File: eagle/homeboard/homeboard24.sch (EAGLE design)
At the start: 124 parts, among them IC1 XCF02S, IC2 25LC080SN, IC3 ATMEGA32U2-TQFP, Q5 BC848SMD, Q6 BC848SMD, Q7 BC848SMD, Q8 BC848SMD, T1 BSS138, T2 BC848, T3 BSS138, U1 XC3S400TQ144, X1 SCART-CLIP, X6 MINI-USB_4P-85-32004-10X, X7 DC21MMX, X8 STEREOJACK

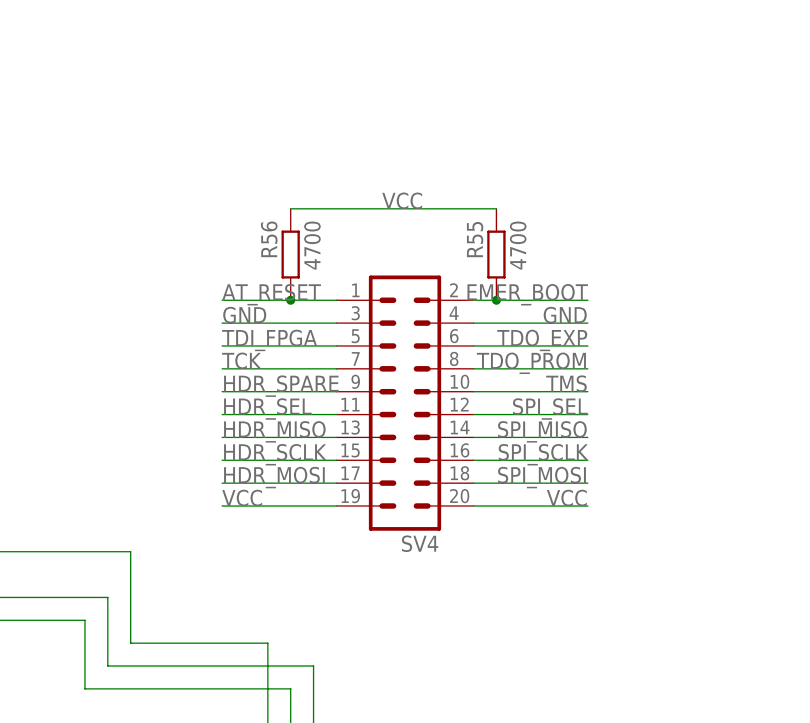
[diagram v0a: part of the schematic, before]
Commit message: moving around
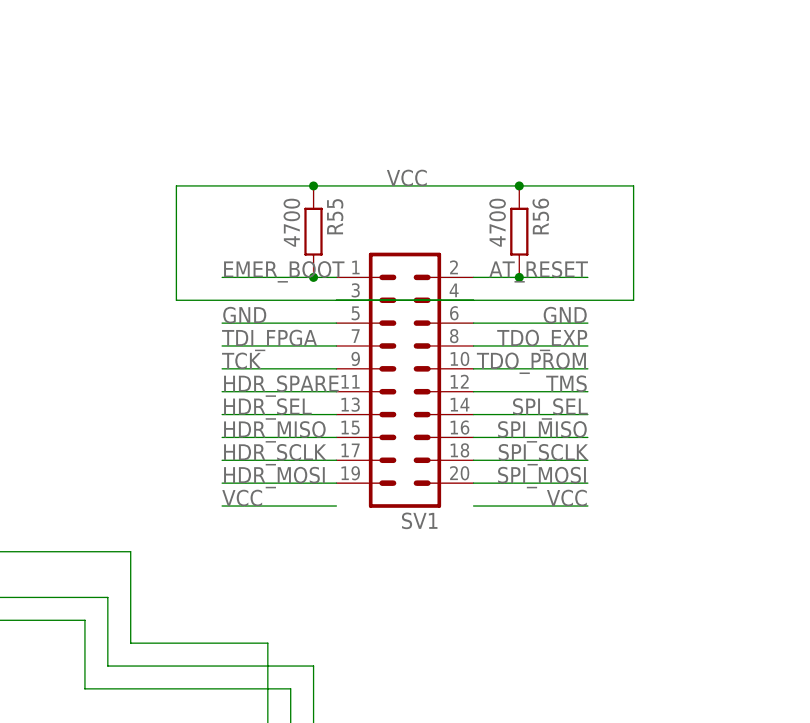
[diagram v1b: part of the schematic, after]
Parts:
- removed SV4: (no value), con-lstb:MA10-2
- added SV1: (no value), con-lstb:MA10-2
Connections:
- net AT_RESET: now also SV1.2; no longer SV4.1
- net EMER_BOOT: now also SV1.1; no longer SV4.2
- net GND: now also SV1.5, SV1.6; no longer SV4.3, SV4.4
- net HDR_MISO: now also SV1.15; no longer SV4.13
- net HDR_MOSI: now also SV1.19; no longer SV4.17
- net HDR_SCLK: now also SV1.17; no longer SV4.15
- net HDR_SEL: now also SV1.13; no longer SV4.11
- net HDR_SPARE: now also SV1.11; no longer SV4.9
- net SPI_MISO: now also SV1.16; no longer SV4.14
- net SPI_MOSI: now also SV1.20; no longer SV4.18
- net SPI_SCLK: now also SV1.18; no longer SV4.16
- net SPI_SEL: now also SV1.14; no longer SV4.12
- net TCK: now also SV1.9; no longer SV4.7
- net TDI_FPGA: now also SV1.7; no longer SV4.5
- net TDO_EXP: now also SV1.8; no longer SV4.6
- net TDO_PROM: now also SV1.10; no longer SV4.8
- net TMS: now also SV1.12; no longer SV4.10
- net VCC: now also SV1.3, SV1.4; no longer SV4.19, SV4.20
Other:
- moved on the sheet: R55, R56
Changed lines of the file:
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@@
 <part name="U$9" library="cpcfpga" deviceset="GNDHOLE" device=""/>
 <part name="SV5" library="con-lstb" deviceset="MA05-2" device=""/>
-<part name="SV4" library="con-lstb" deviceset="MA10-2" device=""/>
 <part name="JP2" library="adafruit" deviceset="PINHD-1X3" device=""/>
 <part name="SV2" library="con-lstb" deviceset="MA03-2" device=""/>
 <part name="SUPPLY16" library="supply2" deviceset="GND" device=""/>
 <part name="C13" library="rcl" deviceset="C-EU" device="C0603" value="100nF"/>
+<part name="SV1" library="con-lstb" deviceset="MA10-2" device="">
+<attribute name="MF" value=""/>
+<attribute name="MPN" value=""/>
+<attribute name="OC_FARNELL" value="unknown"/>
+<attribute name="OC_NEWARK" value="unknown"/>
+</part>
 </parts>
 <sheets>
@@
 <instance part="C41" gate="G$1" x="378.46" y="114.3" rot="R270"/>
 <instance part="SUPPLY22" gate="GND" x="373.38" y="109.22"/>
-<instance part="R55" gate="G$1" x="312.42" y="45.72" rot="MR270"/>
-<instance part="R56" gate="G$1" x="289.56" y="45.72" rot="MR270"/>
+<instance part="R55" gate="G$1" x="292.1" y="48.26" rot="R270"/>
+<instance part="R56" gate="G$1" x="314.96" y="48.26" rot="R270"/>
 <instance part="U$3" gate="G$1" x="541.02" y="40.64"/>
 <instance part="C39" gate="G$1" x="-160.02" y="109.22" smashed="yes">
@@
 <instance part="U$9" gate="G$1" x="-73.66" y="137.16"/>
 <instance part="SV5" gate="G$1" x="76.2" y="-71.12" rot="R180"/>
-<instance part="SV4" gate="G$1" x="302.26" y="30.48" rot="R180"/>
 <instance part="JP2" gate="A" x="330.2" y="119.38" rot="R90"/>
 <instance part="SV2" gate="1" x="289.56" y="-17.78" rot="R90"/>
 <instance part="SUPPLY16" gate="GND" x="292.1" y="-38.1"/>
 <instance part="C13" gate="G$1" x="-93.98" y="109.22"/>
+<instance part="SV1" gate="G$1" x="302.26" y="33.02" rot="R180"/>
 </instances>
 <busses>
@@
 <wire x1="322.58" y1="38.1" x2="309.88" y2="38.1" width="0.1524" layer="91"/>
 <label x="322.58" y="38.1" size="1.778" layer="95" rot="MR0"/>
-<pinref part="SV4" gate="G$1" pin="4"/>
+<pinref part="SV1" gate="G$1" pin="6"/>
 </segment>
 <segment>
 <wire x1="294.64" y1="38.1" x2="281.94" y2="38.1" width="0.1524" layer="91"/>
 <label x="281.94" y="38.1" size="1.778" layer="95"/>
-<pinref part="SV4" gate="G$1" pin="3"/>
+<pinref part="SV1" gate="G$1" pin="5"/>
 </segment>
 <segment>
@@
 <pinref part="R55" gate="G$1" pin="1"/>
 <pinref part="R56" gate="G$1" pin="1"/>
-<wire x1="312.42" y1="50.8" x2="289.56" y2="50.8" width="0.1524" layer="91"/>
-<label x="299.72" y="50.8" size="1.778" layer="95"/>
-</segment>
-<segment>
-<pinref part="SV4" gate="G$1" pin="19"/>
+<wire x1="292.1" y1="53.34" x2="314.96" y2="53.34" width="0.1524" layer="91"/>
+<label x="304.8" y="53.34" size="1.778" layer="95" rot="MR0"/>
+<pinref part="SV1" gate="G$1" pin="3"/>
+<wire x1="294.64" y1="40.64" x2="327.66" y2="40.64" width="0.1524" layer="91"/>
+<wire x1="327.66" y1="40.64" x2="327.66" y2="53.34" width="0.1524" layer="91"/>
+<wire x1="327.66" y1="53.34" x2="314.96" y2="53.34" width="0.1524" layer="91"/>
+<junction x="314.96" y="53.34"/>
+<pinref part="SV1" gate="G$1" pin="4"/>
+<wire x1="309.88" y1="40.64" x2="276.86" y2="40.64" width="0.1524" layer="91"/>
+<wire x1="276.86" y1="40.64" x2="276.86" y2="53.34" width="0.1524" layer="91"/>
+<wire x1="276.86" y1="53.34" x2="292.1" y2="53.34" width="0.1524" layer="91"/>
+<junction x="292.1" y="53.34"/>
+</segment>
+<segment>
 <wire x1="281.94" y1="17.78" x2="294.64" y2="17.78" width="0.1524" layer="91"/>
 <label x="281.94" y="17.78" size="1.778" layer="95"/>
 </segment>
 <segment>
-<pinref part="SV4" gate="G$1" pin="20"/>
 <wire x1="322.58" y1="17.78" x2="309.88" y2="17.78" width="0.1524" layer="91"/>
 <label x="322.58" y="17.78" size="1.778" layer="95" rot="MR0"/>
@@
 <wire x1="281.94" y1="33.02" x2="294.64" y2="33.02" width="0.1524" layer="91"/>
 <label x="281.94" y="33.02" size="1.778" layer="95"/>
-<pinref part="SV4" gate="G$1" pin="7"/>
+<pinref part="SV1" gate="G$1" pin="9"/>
 </segment>
 <segment>
@@
 <label x="322.58" y="30.48" size="1.778" layer="95" rot="MR0"/>
 <wire x1="322.58" y1="30.48" x2="309.88" y2="30.48" width="0.1524" layer="91"/>
-<pinref part="SV4" gate="G$1" pin="10"/>
+<pinref part="SV1" gate="G$1" pin="12"/>
 </segment>
 </net>
@@
 <wire x1="281.94" y1="35.56" x2="294.64" y2="35.56" width="0.1524" layer="91"/>
 <label x="281.94" y="35.56" size="1.778" layer="95"/>
-<pinref part="SV4" gate="G$1" pin="5"/>
+<pinref part="SV1" gate="G$1" pin="7"/>
 </segment>
 </net>
@@
 <segment>
 <wire x1="322.58" y1="22.86" x2="309.88" y2="22.86" width="0.1524" layer="91"/>
-<pinref part="SV4" gate="G$1" pin="16"/>
 <label x="322.58" y="22.86" size="1.778" layer="95" rot="MR0"/>
+<pinref part="SV1" gate="G$1" pin="18"/>
 </segment>
 </net>
@@
 </segment>
 <segment>
-<pinref part="SV4" gate="G$1" pin="18"/>
 <wire x1="322.58" y1="20.32" x2="309.88" y2="20.32" width="0.1524" layer="91"/>
 <label x="322.58" y="20.32" size="1.778" layer="95" rot="MR0"/>
+<pinref part="SV1" gate="G$1" pin="20"/>
 </segment>
 </net>
@@
 </segment>
 <segment>
-<pinref part="SV4" gate="G$1" pin="14"/>
 <wire x1="322.58" y1="25.4" x2="309.88" y2="25.4" width="0.1524" layer="91"/>
 <label x="322.58" y="25.4" size="1.778" layer="95" rot="MR0"/>
+<pinref part="SV1" gate="G$1" pin="16"/>
 </segment>
 </net>
@@
 <wire x1="322.58" y1="27.94" x2="309.88" y2="27.94" width="0.1524" layer="91"/>
 <label x="322.58" y="27.94" size="1.778" layer="95" rot="MR0"/>
-<pinref part="SV4" gate="G$1" pin="12"/>
+<pinref part="SV1" gate="G$1" pin="14"/>
 </segment>
 </net>
@@
 </segment>
 <segment>
-<wire x1="322.58" y1="40.64" x2="312.42" y2="40.64" width="0.1524" layer="91"/>
-<label x="322.58" y="40.64" size="1.778" layer="95" rot="MR0"/>
+<wire x1="281.94" y1="43.18" x2="292.1" y2="43.18" width="0.1524" layer="91"/>
+<label x="281.94" y="43.18" size="1.778" layer="95"/>
 <pinref part="R55" gate="G$1" pin="2"/>
-<wire x1="312.42" y1="40.64" x2="309.88" y2="40.64" width="0.1524" layer="91"/>
-<junction x="312.42" y="40.64"/>
-<pinref part="SV4" gate="G$1" pin="2"/>
+<pinref part="SV1" gate="G$1" pin="1"/>
+<wire x1="292.1" y1="43.18" x2="294.64" y2="43.18" width="0.1524" layer="91"/>
+<junction x="292.1" y="43.18"/>
 </segment>
 </net>
@@
 <wire x1="322.58" y1="33.02" x2="309.88" y2="33.02" width="0.1524" layer="91"/>
 <label x="322.58" y="33.02" size="1.778" layer="95" rot="MR0"/>
-<pinref part="SV4" gate="G$1" pin="8"/>
+<pinref part="SV1" gate="G$1" pin="10"/>
 </segment>
 </net>
@@
 <wire x1="322.58" y1="35.56" x2="309.88" y2="35.56" width="0.1524" layer="91"/>
 <label x="322.58" y="35.56" size="1.778" layer="95" rot="MR0"/>
-<pinref part="SV4" gate="G$1" pin="6"/>
+<pinref part="SV1" gate="G$1" pin="8"/>
 </segment>
 </net>
@@
 </segment>
 <segment>
-<wire x1="281.94" y1="40.64" x2="289.56" y2="40.64" width="0.1524" layer="91"/>
-<label x="281.94" y="40.64" size="1.778" layer="95"/>
+<wire x1="322.58" y1="43.18" x2="314.96" y2="43.18" width="0.1524" layer="91"/>
+<label x="322.58" y="43.18" size="1.778" layer="95" rot="MR0"/>
 <pinref part="R56" gate="G$1" pin="2"/>
-<wire x1="289.56" y1="40.64" x2="294.64" y2="40.64" width="0.1524" layer="91"/>
-<junction x="289.56" y="40.64"/>
-<pinref part="SV4" gate="G$1" pin="1"/>
+<pinref part="SV1" gate="G$1" pin="2"/>
+<wire x1="309.88" y1="43.18" x2="314.96" y2="43.18" width="0.1524" layer="91"/>
+<junction x="314.96" y="43.18"/>
 </segment>
 </net>
@@
 <net name="HDR_MOSI" class="0">
 <segment>
-<pinref part="SV4" gate="G$1" pin="17"/>
 <wire x1="281.94" y1="20.32" x2="294.64" y2="20.32" width="0.1524" layer="91"/>
 <label x="281.94" y="20.32" size="1.778" layer="95"/>
+<pinref part="SV1" gate="G$1" pin="19"/>
 </segment>
 <segment>
@@
 <net name="HDR_SCLK" class="0">
 <segment>
-<pinref part="SV4" gate="G$1" pin="15"/>
 <wire x1="294.64" y1="22.86" x2="281.94" y2="22.86" width="0.1524" layer="91"/>
 <label x="281.94" y="22.86" size="1.778" layer="95"/>
+<pinref part="SV1" gate="G$1" pin="17"/>
 </segment>
 <segment>
@@
 <net name="HDR_MISO" class="0">
 <segment>
-<pinref part="SV4" gate="G$1" pin="13"/>
 <wire x1="281.94" y1="25.4" x2="294.64" y2="25.4" width="0.1524" layer="91"/>
 <label x="281.94" y="25.4" size="1.778" layer="95"/>
+<pinref part="SV1" gate="G$1" pin="15"/>
 </segment>
 <segment>
@@
 <wire x1="281.94" y1="27.94" x2="294.64" y2="27.94" width="0.1524" layer="91"/>
 <label x="281.94" y="27.94" size="1.778" layer="95"/>
-<pinref part="SV4" gate="G$1" pin="11"/>
+<pinref part="SV1" gate="G$1" pin="13"/>
 </segment>
 <segment>
@@
 <wire x1="281.94" y1="30.48" x2="294.64" y2="30.48" width="0.1524" layer="91"/>
 <label x="281.94" y="30.48" size="1.778" layer="95"/>
-<pinref part="SV4" gate="G$1" pin="9"/>
-</segment>
-<segment>
+<pinref part="SV1" gate="G$1" pin="11"/>
+</segment>
+<segment>
